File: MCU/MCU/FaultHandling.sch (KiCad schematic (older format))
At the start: 33 parts, among them Q6 8050, Q7 8050, Q8 8550, Q9 8050

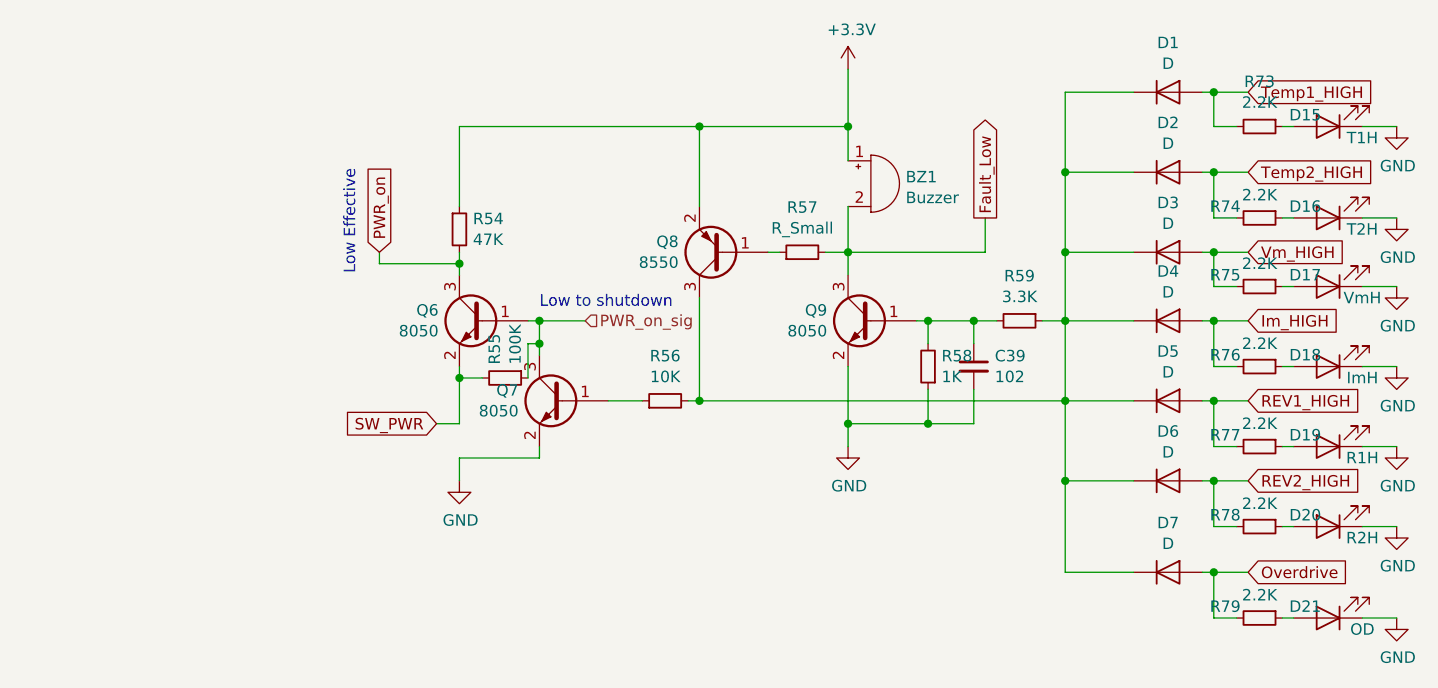
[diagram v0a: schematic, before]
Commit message: Power module
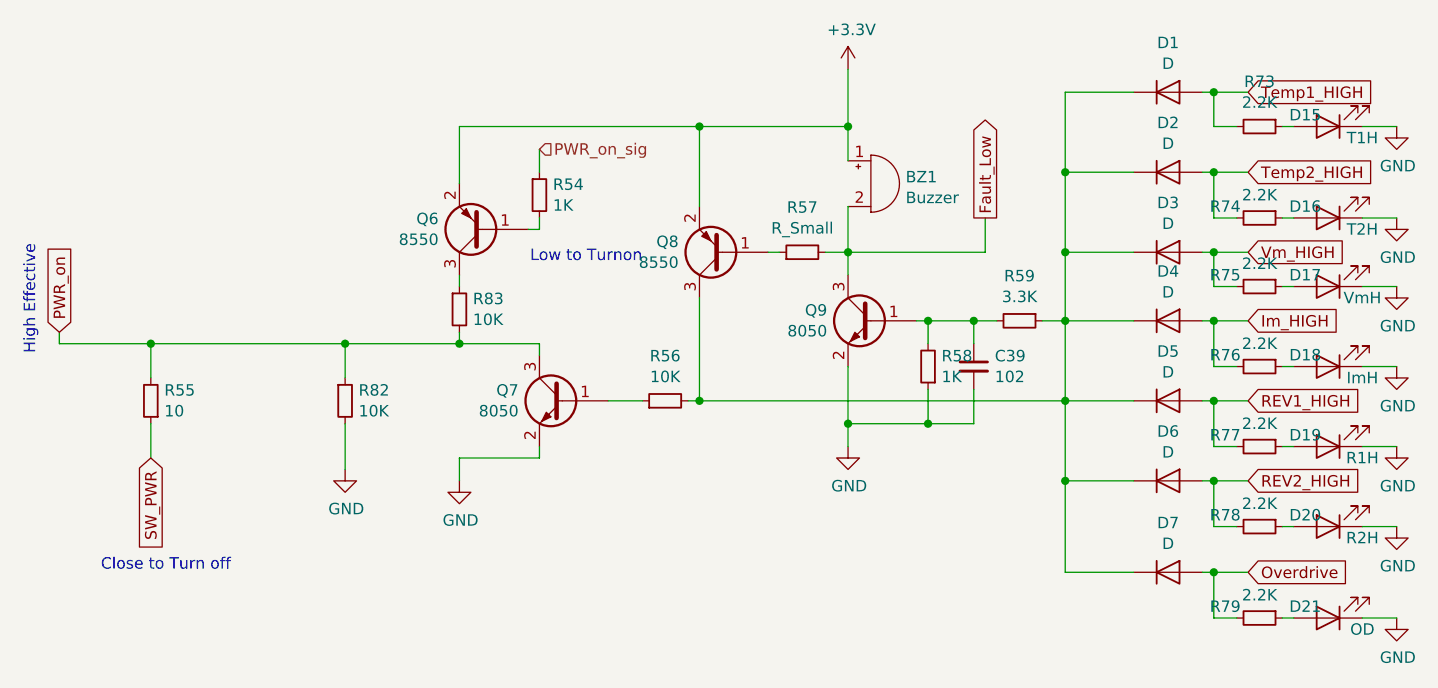
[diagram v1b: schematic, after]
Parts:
- removed Q6: 8050, lc_lib:SOT-23(SOT-23-3), symbol MySchLib:8050
- added Q6: 8550, lc_lib:SOT-23(SOT-23-3), symbol MySchLib:8550
- added R82, R83: 10K, Resistors_SMD:R_0805, symbol Device:R_Small
- R54: value 47K -> 1K
- R55: value 100K -> 10
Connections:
- net +3V3: now also Q6.2 (E); no longer R54.1
- net GND: now also R82.2
- net PWR_on: now also Q7.3 (C), R55.2, R82.1, R83.2; no longer R54.2
- net PWR_on_sig: now also R54.1; no longer Q7.3 (C), R55.1
- net SW_PWR: now also R55.1; no longer R55.2
- new net: Q6.1 (B), R54.2
- new net: Q6.3 (C), R83.1
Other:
- note added: "Close to Turn off"
- note added: "High Effective"
- note added: "Low to Turnon"
- note removed: "Low Effective"
- note removed: "Low to shutdown"
- moved on the sheet: R54, R55
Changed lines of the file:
@@
 Connection ~ 8850 2450
-$Comp
-L MySchLib:8050 Q6
-U 1 1 5EA0931E
-P 6900 2000
-F 0 "Q6" H 7091 2046 50  0000 L CNN
-F 1 "8050" H 7091 1955 50  0000 L CNN
-F 2 "lc_lib:SOT-23(SOT-23-3)" H 7100 1925 50  0001 L CIN
-F 3 "http://www.unisonic.com.tw/datasheet/S8050.pdf" H 6900 2000 50  0001 L CNN
-	1    6900 2000
-	-1   0    0    -1
-$EndComp
 $Comp
 L power:GND #PWR092
@@
 Wire Wire Line
 	6800 2700 6800 2600
-Wire Wire Line
-	6800 1800 6800 1750
-$Comp
-L Device:R_Small R54
-U 1 1 5EA120D3
-P 6800 1600
-F 0 "R54" H 6859 1646 50  0000 L CNN
-F 1 "47K" H 6859 1555 50  0000 L CNN
-F 2 "Resistors_SMD:R_0805" H 6800 1600 50  0001 C CNN
-F 3 "~" H 6800 1600 50  0001 C CNN
-	1    6800 1600
-	1    0    0    -1
-$EndComp
-Text GLabel 6450 1700 1    50   Input ~ 0
+Text GLabel 5050 2050 1    50   Input ~ 0
 PWR_on
-Wire Wire Line
-	7100 2000 7150 2000
 $Comp
 L MySchLib:8050 Q7
@@
 Wire Wire Line
 	7450 2350 7600 2350
-Text Notes 7150 1950 0    50   ~ 0
-Low to shutdown
+Text Notes 7600 1750 2    50   ~ 0
+Low to Turnon
 Wire Wire Line
 	8500 900  8500 1150
-Text GLabel 6700 2450 0    50   Input ~ 0
-SW_PWR
 Text GLabel 9100 1550 1    50   Output ~ 0
 Fault_Low
-Text HLabel 7350 2000 2    50   Input ~ 0
+Text HLabel 7150 1250 2    50   Input ~ 0
 PWR_on_sig
 $Comp
@@
 	-1   0    0    1
 $EndComp
-Text Notes 6350 1800 1    50   ~ 0
-Low Effective
-Wire Wire Line
-	6800 2450 6700 2450
-Wire Wire Line
-	6800 2200 6800 2250
-Wire Wire Line
-	7150 2000 7150 2100
-Connection ~ 6800 2250
-Wire Wire Line
-	6800 2250 6800 2450
-Wire Wire Line
-	7100 2100 7150 2100
-Connection ~ 7150 2100
+Text Notes 4950 2150 1    50   ~ 0
+High Effective
 Wire Wire Line
 	7150 2100 7150 2150
-Wire Wire Line
-	7350 2000 7150 2000
-Connection ~ 7150 2000
 Wire Wire Line
 	9100 1550 9100 1700
@@
 	10100 3100 10250 3100
 Wire Wire Line
-	6450 1700 6450 1750
-Wire Wire Line
-	6450 1750 6800 1750
-Connection ~ 6800 1750
-Wire Wire Line
-	6800 1750 6800 1700
+	5050 2050 5050 2100
 Wire Wire Line
 	6800 1150 7850 1150
-Wire Wire Line
-	6800 1150 6800 1500
 Connection ~ 7850 1150
-Wire Wire Line
-	6900 2250 6800 2250
-Wire Wire Line
-	7100 2250 7100 2100
 $Comp
 L Device:R_Small R55
 U 1 1 5EA1942B
-P 7000 2250
-F 0 "R55" H 6941 2204 50  0000 R CNN
-F 1 "100K" H 6941 2295 50  0000 R CNN
-F 2 "Resistors_SMD:R_0805" H 7000 2250 50  0001 C CNN
-F 3 "~" H 7000 2250 50  0001 C CNN
-	1    7000 2250
-	0    1    1    0
-$EndComp
+P 5450 2350
+F 0 "R55" H 5391 2304 50  0000 R CNN
+F 1 "10" H 5391 2395 50  0000 R CNN
+F 2 "Resistors_SMD:R_0805" H 5450 2350 50  0001 C CNN
+F 3 "~" H 5450 2350 50  0001 C CNN
+	1    5450 2350
+	-1   0    0    1
+$EndComp
+Text GLabel 5450 2600 3    50   Input ~ 0
+SW_PWR
+Wire Wire Line
+	5450 2600 5450 2450
+Wire Wire Line
+	5050 2100 5450 2100
+Wire Wire Line
+	5450 2250 5450 2100
+Connection ~ 5450 2100
+$Comp
+L MySchLib:8550 Q6
+U 1 1 5E5333C0
+P 6900 1600
+F 0 "Q6" H 7091 1554 50  0000 L CNN
+F 1 "8550" H 7091 1645 50  0000 L CNN
+F 2 "lc_lib:SOT-23(SOT-23-3)" H 7100 1525 50  0001 L CIN
+F 3 "http://www.unisonic.com.tw/datasheet/S8550.pdf" H 6900 1600 50  0001 L CNN
+	1    6900 1600
+	-1   0    0    1
+$EndComp
+Wire Wire Line
+	7150 1600 7100 1600
+Text Notes 5800 3100 2    50   ~ 0
+Close to Turn off
+Wire Wire Line
+	7150 1250 7150 1350
+Wire Wire Line
+	7150 1550 7150 1600
+$Comp
+L Device:R_Small R54
+U 1 1 5EA120D3
+P 7150 1450
+F 0 "R54" H 7209 1496 50  0000 L CNN
+F 1 "1K" H 7209 1405 50  0000 L CNN
+F 2 "Resistors_SMD:R_0805" H 7150 1450 50  0001 C CNN
+F 3 "~" H 7150 1450 50  0001 C CNN
+	1    7150 1450
+	1    0    0    -1
+$EndComp
+$Comp
+L Device:R_Small R83
+U 1 1 5E55F9C9
+P 6800 1950
+F 0 "R83" H 6859 1996 50  0000 L CNN
+F 1 "10K" H 6859 1905 50  0000 L CNN
+F 2 "Resistors_SMD:R_0805" H 6800 1950 50  0001 C CNN
+F 3 "~" H 6800 1950 50  0001 C CNN
+	1    6800 1950
+	1    0    0    -1
+$EndComp
+Wire Wire Line
+	6800 1850 6800 1800
+Wire Wire Line
+	6800 2050 6800 2100
+Connection ~ 6800 2100
+Wire Wire Line
+	6800 2100 7150 2100
+Wire Wire Line
+	6800 1400 6800 1150
+Wire Wire Line
+	5450 2100 6300 2100
+$Comp
+L Device:R_Small R82
+U 1 1 5E57489E
+P 6300 2350
+F 0 "R82" H 6359 2396 50  0000 L CNN
+F 1 "10K" H 6359 2305 50  0000 L CNN
+F 2 "Resistors_SMD:R_0805" H 6300 2350 50  0001 C CNN
+F 3 "~" H 6300 2350 50  0001 C CNN
+	1    6300 2350
+	1    0    0    -1
+$EndComp
+Wire Wire Line
+	6300 2250 6300 2100
+Connection ~ 6300 2100
+Wire Wire Line
+	6300 2100 6800 2100
+$Comp
+L power:GND #PWR0153
+U 1 1 5E5779FA
+P 6300 2650
+F 0 "#PWR0153" H 6300 2400 50  0001 C CNN
+F 1 "GND" H 6305 2477 50  0000 C CNN
+F 2 "" H 6300 2650 50  0001 C CNN
+F 3 "" H 6300 2650 50  0001 C CNN
+	1    6300 2650
+	1    0    0    -1
+$EndComp
+Wire Wire Line
+	6300 2450 6300 2650
 $EndSCHEMATC
